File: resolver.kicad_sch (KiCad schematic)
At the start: 17 parts

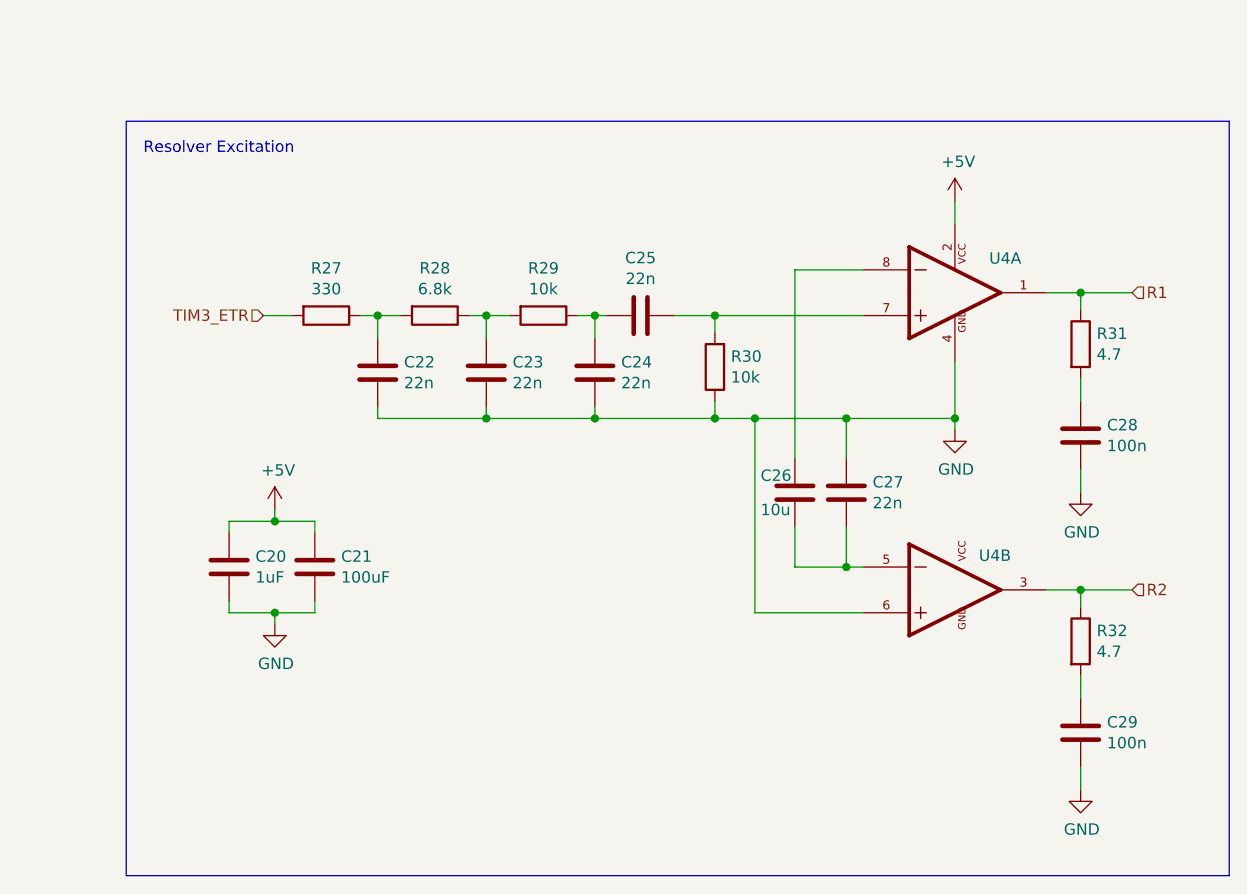
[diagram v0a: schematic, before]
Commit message: started adding AD2S
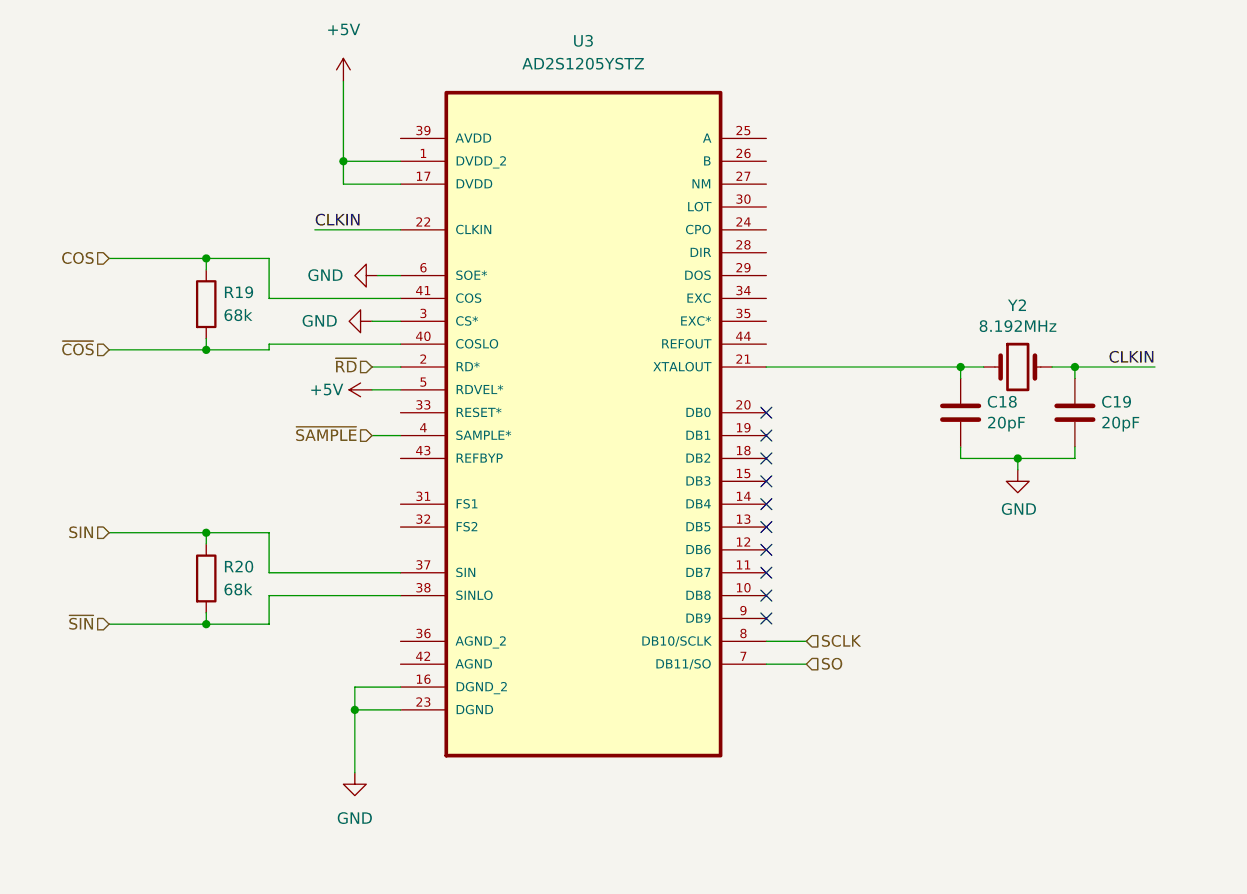
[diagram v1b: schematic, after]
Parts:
- removed C20: 1uF, Capacitor_SMD:C_0603_1608Metric, symbol prius_gen2-rescue:C-Device-prius_gen2-rescue
- removed C21: 100uF, Capacitor_SMD:C_Elec_6.3x7.7, symbol prius_gen2-rescue:C-Device-prius_gen2-rescue
- removed C22, C23, C24, C25, C27: 22n, Capacitor_SMD:C_0603_1608Metric, symbol prius_gen2-rescue:C-Device-prius_gen2-rescue
- removed C26: 10u, Capacitor_SMD:C_0603_1608Metric, symbol prius_gen2-rescue:C-Device-prius_gen2-rescue
- removed C28, C29: 100n, Capacitor_SMD:C_0603_1608Metric, symbol prius_gen2-rescue:C-Device-prius_gen2-rescue
- removed R27: 330, Resistor_SMD:R_0603_1608Metric, symbol prius_gen2-rescue:R-Device-prius_gen2-rescue
- removed R28: 6.8k, Resistor_SMD:R_0603_1608Metric, symbol prius_gen2-rescue:R-Device-prius_gen2-rescue
- removed R29, R30: 10k, Resistor_SMD:R_0603_1608Metric, symbol prius_gen2-rescue:R-Device-prius_gen2-rescue
- removed R31, R32: 4.7, Resistor_SMD:R_0603_1608Metric, symbol prius_gen2-rescue:R-Device-prius_gen2-rescue
- removed U4: (no value), symbol prius_gen2-rescue:TDA2822D-TDA2822D-prius_gen2-rescue
- added C18, C19: 20pF, Capacitor_SMD:C_0603_1608Metric, symbol Device:C
- added R19, R20: 68k, symbol Device:R
- added U3: AD2S1205YSTZ, QFP80P1200X1200X160-44N, symbol AD2S1205YSTZ:AD2S1205YSTZ
- added Y2: 8.192MHz, Crystal:Crystal_SMD_5032-2Pin_5.0x3.2mm, symbol Device:Crystal
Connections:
- net +5V: now also U3.1 (DVDD_2), U3.17 (DVDD), U3.5 (RDVEL*)
- net GND: now also C18.1, C19.1, U3.16 (DGND_2), U3.23 (DGND), U3.3 (CS*), U3.6 (SOE*)
- new net: C18.2, U3.21 (XTALOUT), Y2.1
- new net CLKIN: C19.2, U3.22 (CLKIN), Y2.2
- new net COS: R19.1, U3.41 (COS)
- new net SCLK: U3.8 (DB10/SCLK)
- new net SIN: R20.1, U3.37 (SIN)
- new net SO: U3.7 (DB11/SO)
- new net ~{COS}: R19.2, U3.40 (COSLO)
- new net ~{RD}: U3.2 (RD*)
- new net ~{SAMPLE}: U3.4 (SAMPLE*)
- new net ~{SIN}: R20.2, U3.38 (SINLO)
- no-connect marks 0 -> 10
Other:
- note removed: "Resolver Excitation"
